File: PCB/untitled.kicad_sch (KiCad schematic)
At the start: 17 parts, among them J2 Conn_01x02_Pin, J3 Conn_01x02_Pin, J4 Conn_01x03_Pin, J5 Conn_01x03_Pin, J6 Conn_01x03_Pin, J7 Conn_01x07_Pin, J8 Conn_01x08_Socket, U2 MPU-6050

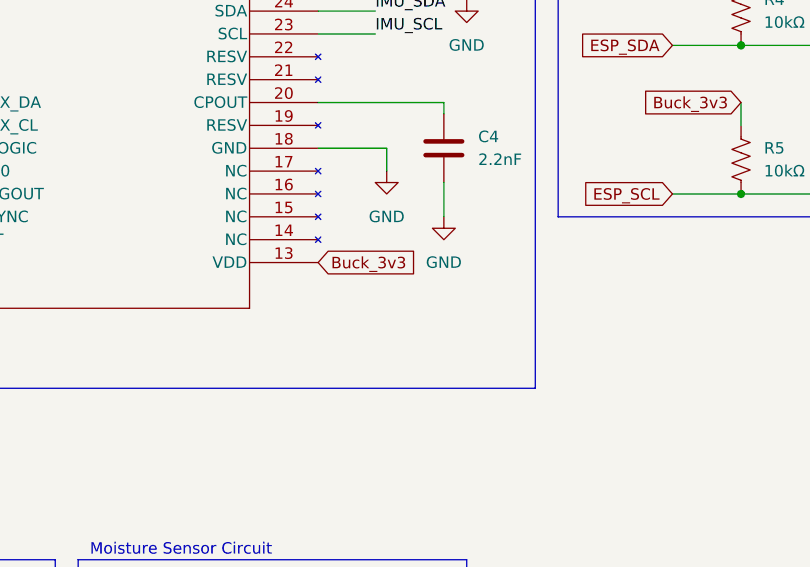
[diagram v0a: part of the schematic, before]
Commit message: She buck on my converter till I 3.3V DC
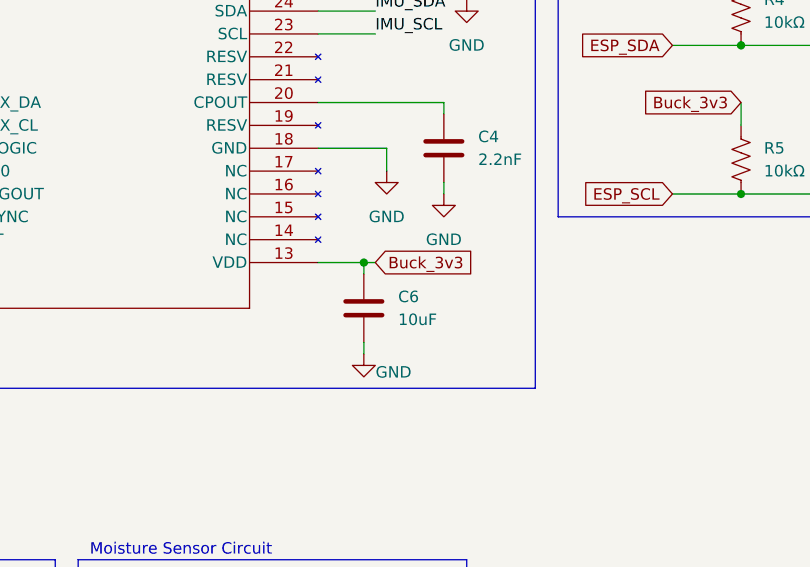
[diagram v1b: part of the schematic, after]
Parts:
- added C6: 10uF, symbol Device:C
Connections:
- net Buck_3v3: now also C6.1
- net GND: now also C6.2
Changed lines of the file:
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@@
+	)
+	(junction
+		(at 86.36 60.96)
+		(diameter 0)
+		(color 0 0 0 0)
 	)
 	(junction
@@
 	(wire
 		(pts
+			(xy 86.36 60.96) (xy 86.36 62.23)
+		)
+		(stroke
+			(width 0)
+			(type default)
+		)
+	)
+	(wire
+		(pts
 			(xy 31.75 153.67) (xy 36.83 153.67)
 		)
@@
 	(wire
 		(pts
+			(xy 87.63 60.96) (xy 86.36 60.96)
+		)
+		(stroke
+			(width 0)
+			(type default)
+		)
+	)
+	(wire
+		(pts
 			(xy 21.59 62.23) (xy 21.59 66.04)
 		)
@@
 	(wire
 		(pts
+			(xy 86.36 69.85) (xy 86.36 71.12)
+		)
+		(stroke
+			(width 0)
+			(type default)
+		)
+	)
+	(wire
+		(pts
 			(xy 76.2 107.95) (xy 76.2 115.57)
 		)
@@
 	(wire
 		(pts
-			(xy 95.25 52.07) (xy 95.25 55.88)
+			(xy 95.25 52.07) (xy 95.25 53.34)
+		)
+		(stroke
+			(width 0)
+			(type default)
+		)
+	)
+	(wire
+		(pts
+			(xy 86.36 60.96) (xy 81.28 60.96)
 		)
 		(stroke
@@
 	(global_label "Buck_3v3"
 		(shape input)
-		(at 81.28 60.96 0)
+		(at 87.63 60.96 0)
 		(fields_autoplaced yes)
 		(effects
@@
 		)
 		(property "Intersheetrefs" "${INTERSHEET_REFS}"
-			(at 93.1551 60.96 0)
+			(at 99.5051 60.96 0)
 			(effects
 				(font
@@
 	(symbol
 		(lib_id "power:GND")
-		(at 95.25 55.88 0)
+		(at 95.25 53.34 0)
 		(unit 1)
 		(exclude_from_sim no)
@@
 		(fields_autoplaced yes)
 		(property "Reference" "#PWR09"
-			(at 95.25 62.23 0)
+			(at 95.25 59.69 0)
 			(effects
 				(font
@@
 		)
 		(property "Value" "GND"
-			(at 95.25 60.96 0)
+			(at 95.25 58.42 0)
 			(effects
 				(font
@@
 		)
 		(property "Footprint" ""
-			(at 95.25 55.88 0)
+			(at 95.25 53.34 0)
 			(effects
 				(font
@@
 		)
 		(property "Datasheet" ""
-			(at 95.25 55.88 0)
+			(at 95.25 53.34 0)
 			(effects
 				(font
@@
 		)
 		(property "Description" "Power symbol creates a global label with name \"GND\" , ground"
-			(at 95.25 55.88 0)
+			(at 95.25 53.34 0)
 			(effects
 				(font
@@
 	)
 	(symbol
+		(lib_id "Device:C")
+		(at 86.36 66.04 0)
+		(unit 1)
+		(exclude_from_sim no)
+		(in_bom yes)
+		(on_board yes)
+		(dnp no)
+		(fields_autoplaced yes)
+		(property "Reference" "C6"
+			(at 90.17 64.7699 0)
+			(effects
+				(font
+					(size 1.27 1.27)
+				)
+				(justify left)
+			)
+		)
+		(property "Value" "10uF"
+			(at 90.17 67.3099 0)
+			(effects
+				(font
+					(size 1.27 1.27)
+				)
+				(justify left)
+			)
+		)
+		(property "Footprint" ""
+			(at 87.3252 69.85 0)
+			(effects
+				(font
+					(size 1.27 1.27)
+				)
+				(hide yes)
+			)
+		)
+		(property "Datasheet" "~"
+			(at 86.36 66.04 0)
+			(effects
+				(font
+					(size 1.27 1.27)
+				)
+				(hide yes)
+			)
+		)
+		(property "Description" "Unpolarized capacitor"
+			(at 86.36 66.04 0)
+			(effects
+				(font
+					(size 1.27 1.27)
+				)
+				(hide yes)
+			)
+		)
+		(pin "1"
+		)
+		(pin "2"
+		)
+		(instances
+			(project "Smart_Backpack"
+				(path "/38abc652-c887-4ef7-a45f-d93ca7f4b2d6/d6ce3c21-a733-4fa1-8134-cea10a02c4e5"
+					(reference "C6")
+					(unit 1)
+				)
+			)
+		)
+	)
+	(symbol
 		(lib_id "power:+3V3")
 		(at 48.26 120.65 0)
@@
 					(unit 1)
 				)
+			)
+		)
+	)
+	(symbol
+		(lib_id "power:GND")
+		(at 86.36 71.12 0)
+		(unit 1)
+		(exclude_from_sim no)
+		(in_bom yes)
+		(on_board yes)
+		(dnp no)
+		(property "Reference" "#PWR024"
+			(at 86.36 77.47 0)
+			(effects
+				(font
+					(size 1.27 1.27)
+				)
+				(hide yes)
+			)
+		)
+		(property "Value" "GND"
+			(at 89.662 73.152 0)
+			(effects
+				(font
+					(size 1.27 1.27)
+				)
+			)
+		)
+		(property "Footprint" ""
+			(at 86.36 71.12 0)
+			(effects
+				(font
+					(size 1.27 1.27)
+				)
+				(hide yes)
+			)
+		)
+		(property "Datasheet" ""
+			(at 86.36 71.12 0)
+			(effects
+				(font
+					(size 1.27 1.27)
+				)
+				(hide yes)
+			)
+		)
+		(property "Description" "Power symbol creates a global label with name \"GND\" , ground"
+			(at 86.36 71.12 0)
+			(effects
+				(font
+					(size 1.27 1.27)
+				)
+				(hide yes)
+			)
+		)
+		(pin "1"
+		)
+		(instances
+			(project "Smart_Backpack"
+				(path "/38abc652-c887-4ef7-a45f-d93ca7f4b2d6/d6ce3c21-a733-4fa1-8134-cea10a02c4e5"
+					(reference "#PWR024")
+					(unit 1)
+				)
